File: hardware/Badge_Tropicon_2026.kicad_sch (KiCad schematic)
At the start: 56 parts, among them J1 Battery, P1 USB_C_Plug_USB2.0, Q1 DMG3415U-7, SW3 ON, U1 ESP32-S3-WROOM-1-N8, U2 BL8072CLTR33, U3 Si4463, U4 AHT30, U5 VGdd79S915N0S1, Y1 30MHz

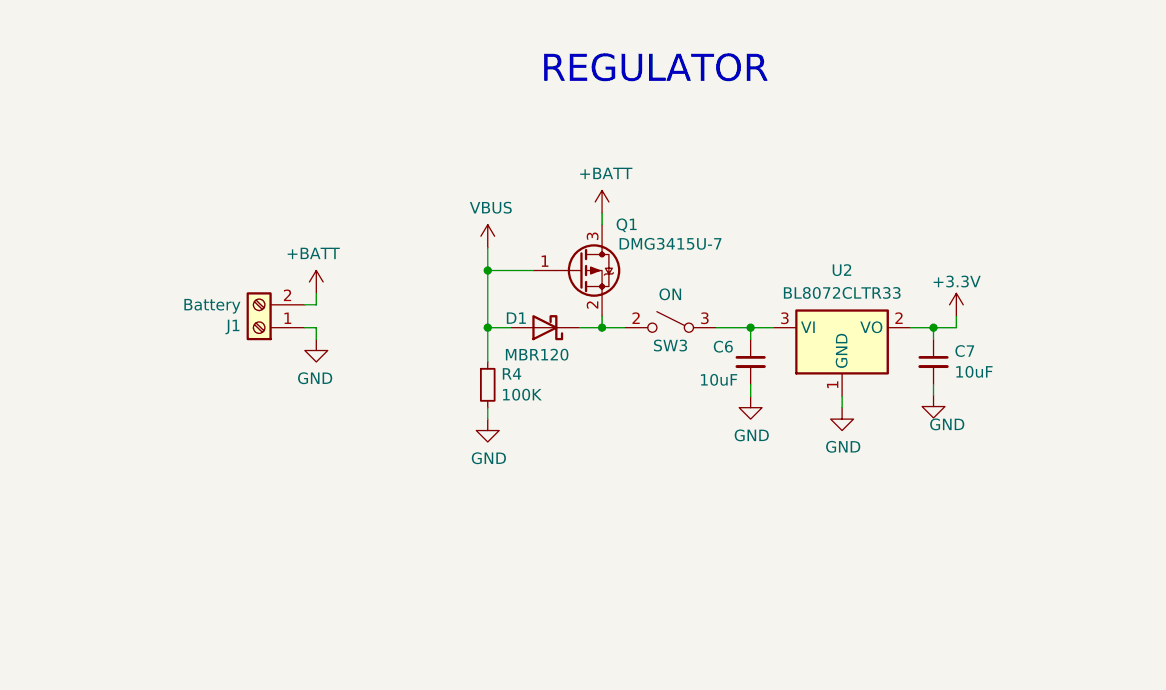
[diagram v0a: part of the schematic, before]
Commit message: feat(Hw):Update_BOM
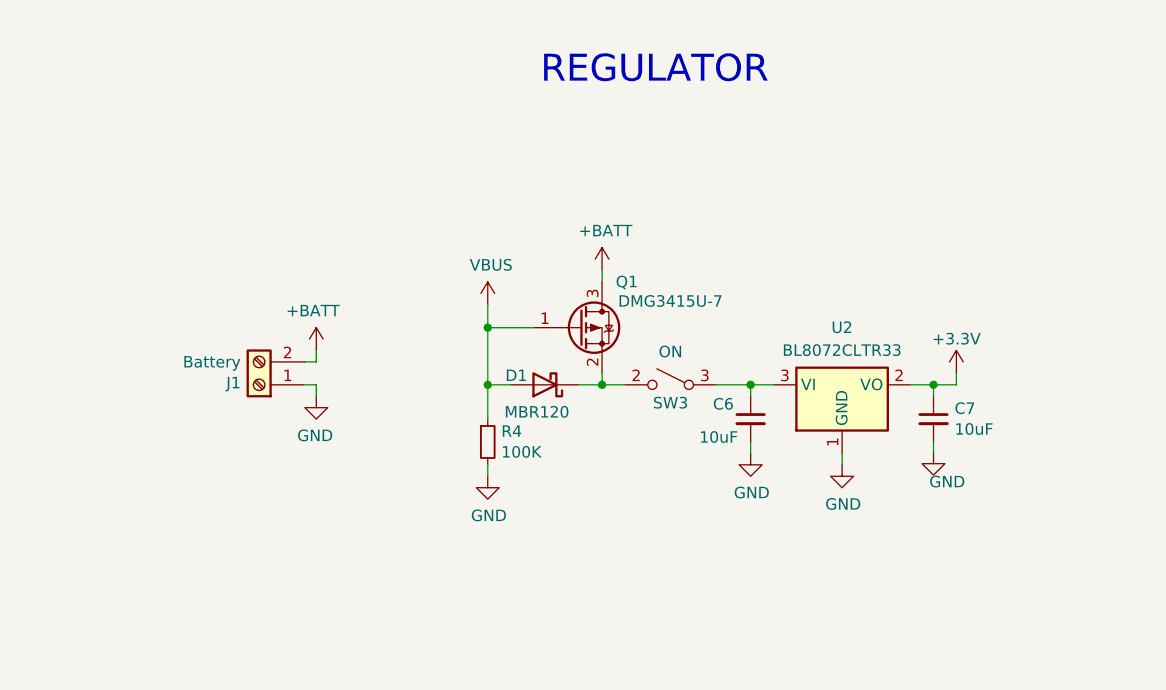
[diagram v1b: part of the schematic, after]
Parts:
- AE1: footprint (none) -> Footprints:SMA_EDGE; LCSC# (none) -> C530661
- U1: footprint (none) -> Footprints:ESP32-S3-WROOM-1_EXP
- U4: footprint (none) -> Footprints:AHT30
- Y1: footprint (none) -> Crystal:Crystal_SMD_Abracon_ABM8G-4Pin_3.2x2.5mm
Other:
- moved on the sheet: C6, C7, D1, J1, Q1, R4, SW3, U2
